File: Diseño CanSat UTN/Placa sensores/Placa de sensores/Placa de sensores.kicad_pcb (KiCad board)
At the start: 2 copper layers, 60 x 60 mm, 6 parts, among them J1 Conn_01x15_MountingPin, J2 Conn_01x15_MountingPin, U1 BMP280

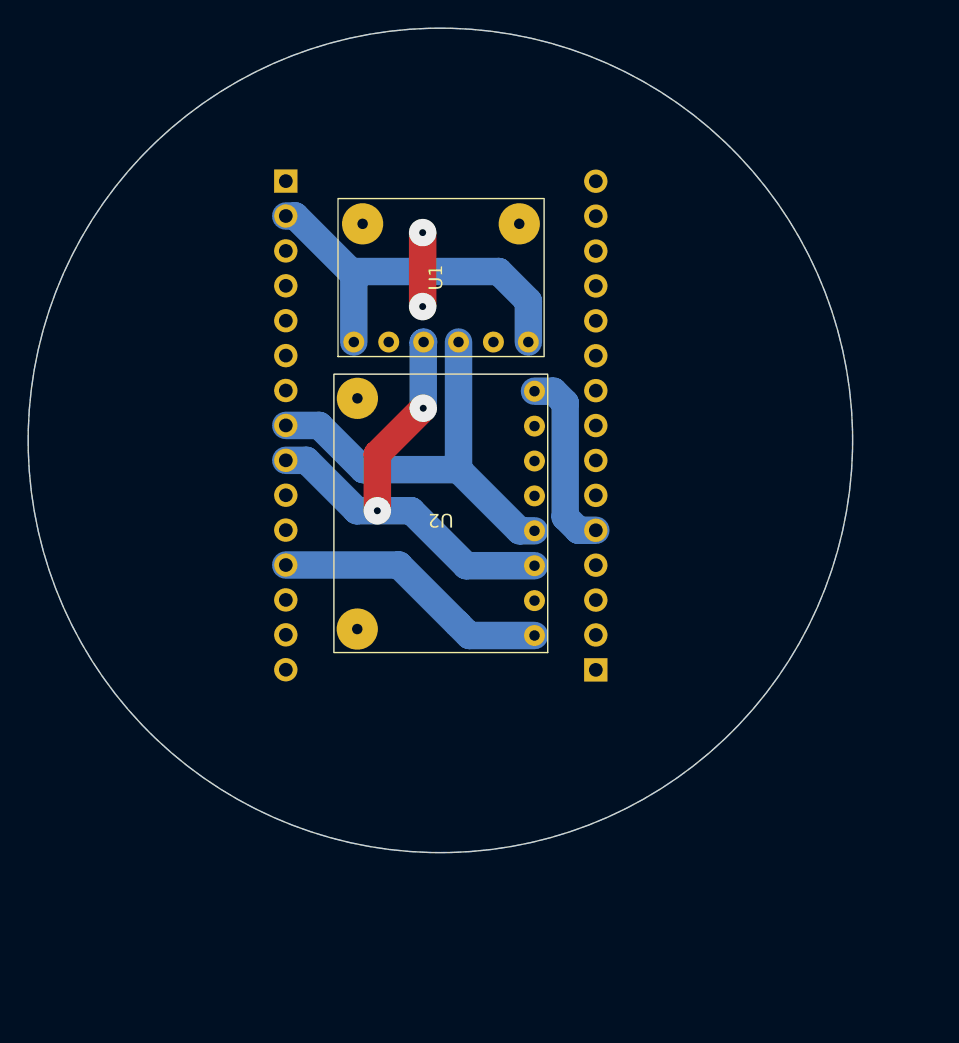
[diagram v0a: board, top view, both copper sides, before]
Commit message: ACTUALIZACION
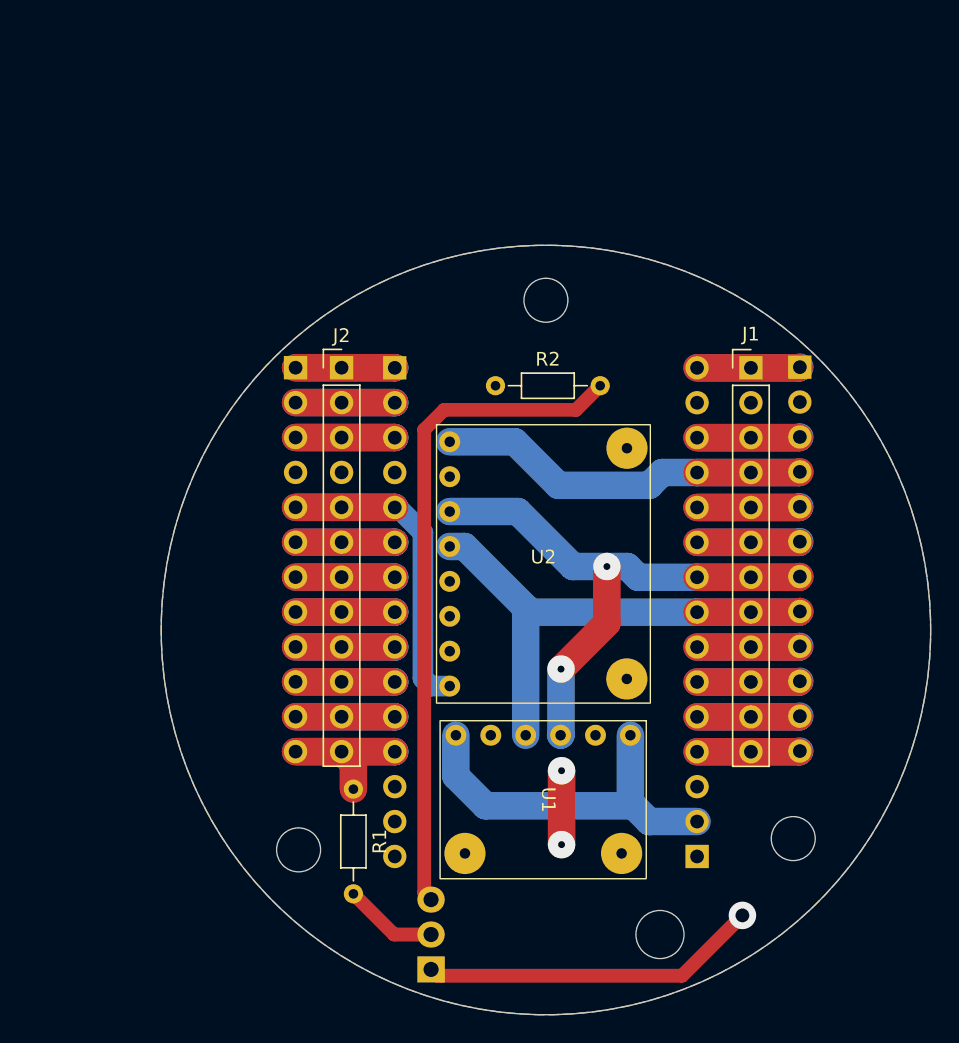
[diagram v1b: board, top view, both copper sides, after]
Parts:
- added ?: , , F.Cu at (130.8, 108.8)
- added ?: , , F.Cu at (167.5, 83.4)
- added ?: , , F.Cu at (167.5, 106.3)
- added ?: , , F.Cu at (167.5, 98.7)
- added ?: , , F.Cu at (130.8, 96.2)
- added ?: , , F.Cu at (167.5, 88.5)
- added ?: , , F.Cu at (130.8, 98.7)
- added ?: , , F.Cu at (167.5, 80.9)
- added ?: , , F.Cu at (130.8, 86.0)
- added ?: , , F.Cu at (130.8, 93.6)
- added ?: , , F.Cu at (167.5, 86.0)
- added ?: , , F.Cu at (167.5, 108.8)
- added ?: , , F.Cu at (130.8, 101.2)
- added ?: , , F.Cu at (167.5, 101.2)
- added ?: , , F.Cu at (130.8, 88.5)
- added ?: , , F.Cu at (167.5, 103.7)
- added ?: , , F.Cu at (167.5, 96.1)
- added ?: , , F.Cu at (167.5, 91.0)
- added ?: , , F.Cu at (130.8, 106.3)
- added ?: , , F.Cu at (130.8, 80.9)
- added ?: , , F.Cu at (130.8, 91.1)
- added ?: , , F.Cu at (130.8, 103.8)
- added ?: , , F.Cu at (167.5, 93.6)
- added ?: , , F.Cu at (130.8, 83.5)
- added J1: Conn_01x15_MountingPin, Connector_PinHeader_2.54mm:PinHeader_1x15_P2.54mm_Vertical, F.Cu at (163.9, 80.9)
- added J2: Conn_01x15_MountingPin, Connector_PinHeader_2.54mm:PinHeader_1x15_P2.54mm_Vertical, F.Cu at (134.1, 80.9)
- added Q1: NPN, Package_TO_SOT_THT:TO-220-3_Horizontal_TabDown, B.Cu at (140.6, 124.7)
- added R1: R, Resistor_THT:R_Axial_DIN0204_L3.6mm_D1.6mm_P7.62mm_Horizontal, F.Cu at (135.0, 111.6)
- added R2: R, Resistor_THT:R_Axial_DIN0204_L3.6mm_D1.6mm_P7.62mm_Horizontal, F.Cu at (145.3, 82.2)
- added REF**: MountingHole_3.2mm_M3, MountingHole:MountingHole_3.2mm_M3, F.Cu at (167.0, 115.2)
- added REF**: MountingHole_3.2mm_M3, MountingHole:MountingHole_3.2mm_M3, F.Cu at (131.0, 116.0)
- added REF**: MountingHole_3.2mm_M3, MountingHole:MountingHole_3.2mm_M3, F.Cu at (149.0, 76.0)
- moved J1 57.5 mm to (160.0, 116.5), turned to 0 degrees
- moved ? 49.5 mm to (154.5, 116.3), turned to 180 degrees
- moved ? 46.0 mm to (143.1, 116.3), turned to 180 degrees
- moved U1 38.7 mm to (148.7, 112.3), turned to -90 degrees
- moved J2 26.4 mm to (138.0, 80.9), turned to 180 degrees
- moved U2 8.33 mm to (148.8, 95.2), turned to 0 degrees
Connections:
- J1 pad 12: /27 -> Net-(Q1-E)
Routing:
- net Net-(Q1-E): track 0.00 -> 83.2 mm
- net +9V: track 0.00 -> 24.7 mm, vias 0 -> 1
- net /27: track 20.2 -> 0.00 mm
- net /12: track 0.00 -> 17.5 mm
- net /5: track 13.5 -> 30.0 mm
- net /25: track 0.00 -> 15.0 mm
- net /30: track 0.00 -> 15.0 mm
- net /28: track 0.00 -> 15.0 mm
- net /26: track 0.00 -> 15.0 mm
- net /22: track 0.00 -> 15.0 mm
- net /21: track 0.00 -> 15.0 mm
- net /20: track 0.00 -> 15.0 mm
- net /19: track 0.00 -> 15.0 mm
- net /8: track 0.00 -> 14.4 mm
- net /6: track 0.00 -> 14.4 mm
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- added copper zone on F.Cu, net GND
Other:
- board size 60 x 60 mm -> 56 x 56 mm
